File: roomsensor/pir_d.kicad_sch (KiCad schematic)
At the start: 2 parts, among them U1301 SM03B-SRSS-TB(LF)(SN)(P)

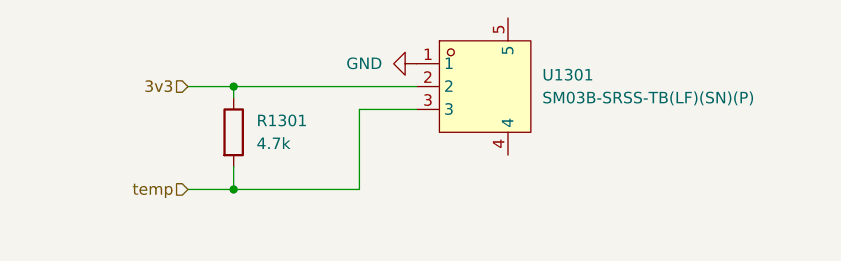
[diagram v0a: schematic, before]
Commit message: sensor v2.1
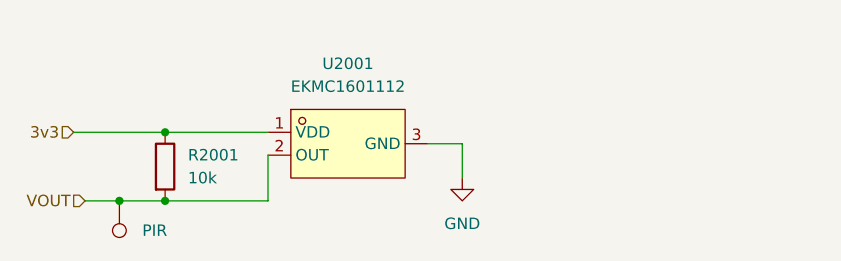
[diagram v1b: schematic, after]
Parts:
- removed R1301: 4.7k, Resistor_SMD:R_0603_1608Metric, symbol Device:R
- removed U1301: SM03B-SRSS-TB(LF)(SN)(P), easyeda2kicad:CONN-SMD_SM03B-SRSS-TB-LF-SN-P, symbol easyeda2kicad:SM03B-SRSS-TB(LF)(SN)(P)
- added R2001: 10k, Resistor_SMD:R_0603_1608Metric, symbol Device:R
- added TP1901: LabeledTestPoint, easyeda2kicad:LabeledTestPoint, symbol easyeda2kicad:LabeledTestPoint
- added U2001: EKMC1601112, easyeda2kicad:SENSOR-TH_EKMC1601111, symbol easyeda2kicad:EKMC1601112
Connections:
- net 3v3: now also R2001.1, U2001.1 (VDD)
- net GND: now also U2001.3 (GND)
- new net VOUT: R2001.2, TP1901.1, U2001.2 (OUT)
